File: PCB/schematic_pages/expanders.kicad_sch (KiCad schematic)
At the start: 32 parts

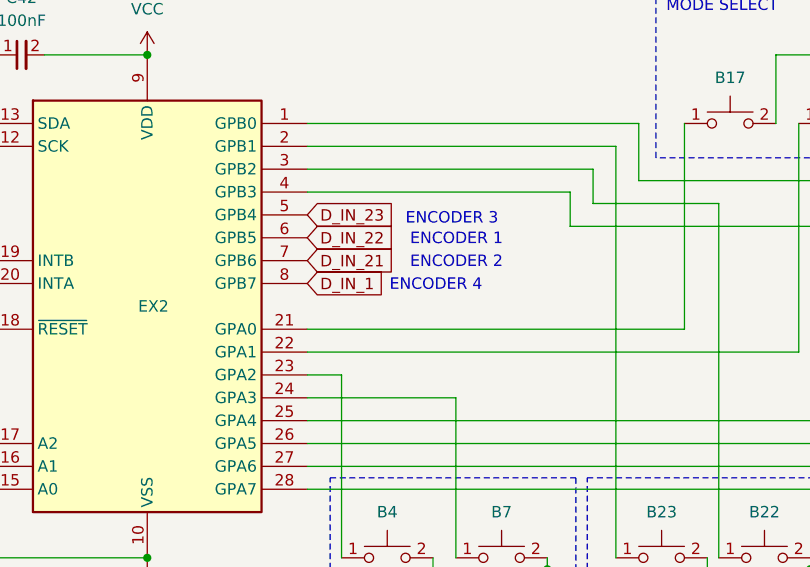
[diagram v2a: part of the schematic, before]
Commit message: PCB V1.0 DONE
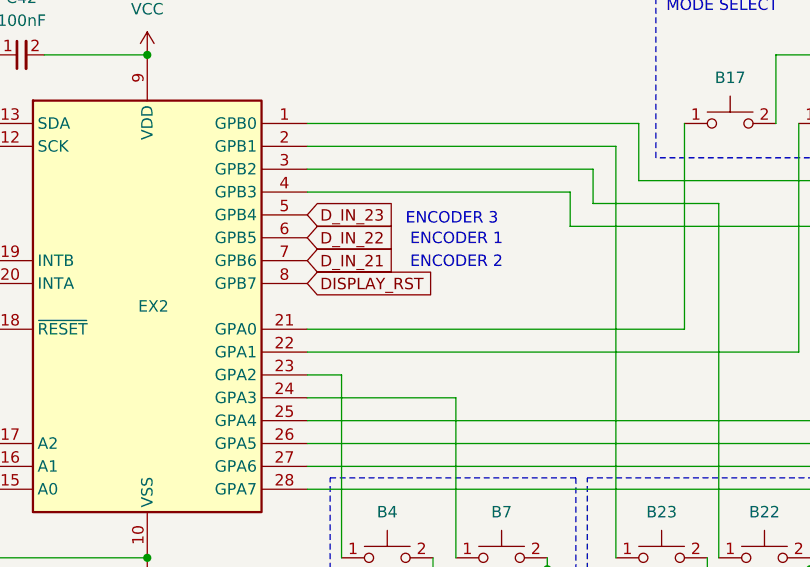
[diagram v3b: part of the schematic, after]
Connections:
- net D_IN_1 renamed DISPLAY_RST
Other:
- note removed: "ENCODER 4"
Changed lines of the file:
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@@
-		)
-	)
-	(text "ENCODER 4"
-		(exclude_from_sim no)
-		(at 112.014 122.174 0)
-		(effects
-			(font
-				(size 1.27 1.27)
-			)
-			(justify left)
 		)
 	)
@@
 			(width 0)
 			(type default)
-		)
-	)
-	(global_label "D_IN_1"
-		(shape input)
-		(at 102.87 121.92 0)
-		(fields_autoplaced yes)
-		(effects
-			(font
-				(size 1.27 1.27)
-				(color 221 133 0 1)
-			)
-			(justify left)
-		)
-		(property "Intersheetrefs" "${INTERSHEET_REFS}"
-			(at 112.2052 121.92 0)
-			(effects
-				(font
-					(size 1.27 1.27)
-				)
-				(justify left)
-				(hide yes)
-			)
 		)
 	)
@@
 			(effects
 				(font
+					(size 1.27 1.27)
+				)
+				(justify left)
+				(hide yes)
+			)
+		)
+	)
+	(global_label "DISPLAY_RST"
+		(shape input)
+		(at 102.87 121.92 0)
+		(fields_autoplaced yes)
+		(effects
+			(font
+				(size 1.27 1.27)
+				(color 221 133 0 1)
+			)
+			(justify left)
+		)
+		(property "Intersheetrefs" "${INTERSHEET_REFS}"
+			(at 117.8295 121.92 0)
+			(effects
+				(font
